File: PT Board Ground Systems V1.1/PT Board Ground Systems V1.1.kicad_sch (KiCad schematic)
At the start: 9 parts, among them J1 POWER IN, J2 OUT CHAN A, J3 OUT CHAN B

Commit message: Changed all the things to 5mm pitch
yuck big board be like
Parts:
- J1: footprint TerminalBlock_Phoenix:TerminalBlock_Phoenix_MPT-0,5-2-2.54_1x02_P2.54mm_Horizontal -> TerminalBlock_Phoenix:TerminalBlock_Phoenix_PT-1,5-2-5.0-H_1x02_P5.00mm_Horizontal
- J2, J3: footprint TerminalBlock_Phoenix:TerminalBlock_Phoenix_MPT-0,5-8-2.54_1x08_P2.54mm_Horizontal -> TerminalBlock_Phoenix:TerminalBlock_Phoenix_PT-1,5-8-5.0-H_1x08_P5.00mm_Horizontal

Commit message: Woek
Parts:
- J1: footprint TerminalBlock_Phoenix:TerminalBlock_Phoenix_PT-1,5-2-5.0-H_1x02_P5.00mm_Horizontal -> TerminalBlock_Phoenix:TerminalBlock_Phoenix_PT-1,5-2-3.5-H_1x02_P3.50mm_Horizontal
- J2, J3: footprint TerminalBlock_Phoenix:TerminalBlock_Phoenix_PT-1,5-8-5.0-H_1x08_P5.00mm_Horizontal -> TerminalBlock_Phoenix:TerminalBlock_Phoenix_PT-1,5-8-3.5-H_1x08_P3.50mm_Horizontal
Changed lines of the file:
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@@
       (effects (font (size 1.27 1.27)))
     )
-    (property "Footprint" "TerminalBlock_Phoenix:TerminalBlock_Phoenix_PT-1,5-2-5.0-H_1x02_P5.00mm_Horizontal" (at 20.32 30.48 0)
+    (property "Footprint" "TerminalBlock_Phoenix:TerminalBlock_Phoenix_PT-1,5-2-3.5-H_1x02_P3.50mm_Horizontal" (at 20.32 30.48 0)
       (effects (font (size 1.27 1.27)) hide)
     )
@@
       (effects (font (size 1.27 1.27)))
     )
-    (property "Footprint" "TerminalBlock_Phoenix:TerminalBlock_Phoenix_PT-1,5-8-5.0-H_1x08_P5.00mm_Horizontal" (at 53.34 19.685 0)
+    (property "Footprint" "TerminalBlock_Phoenix:TerminalBlock_Phoenix_PT-1,5-8-3.5-H_1x08_P3.50mm_Horizontal" (at 53.34 19.685 0)
       (effects (font (size 1.27 1.27)) hide)
     )
@@
       (effects (font (size 1.27 1.27)))
     )
-    (property "Footprint" "TerminalBlock_Phoenix:TerminalBlock_Phoenix_PT-1,5-8-5.0-H_1x08_P5.00mm_Horizontal" (at 74.93 19.685 0)
-      (effects (font (size 1.27 1.27)) hide)
-    )
+    (property "Footprint" "TerminalBlock_Phoenix:TerminalBlock_Phoenix_PT-1,5-8-3.5-H_1x08_P3.50mm_Horizontal" (at 74.93 19.685 0)
+      (effects (font (size 1.27 1.27)) hide)
+    )

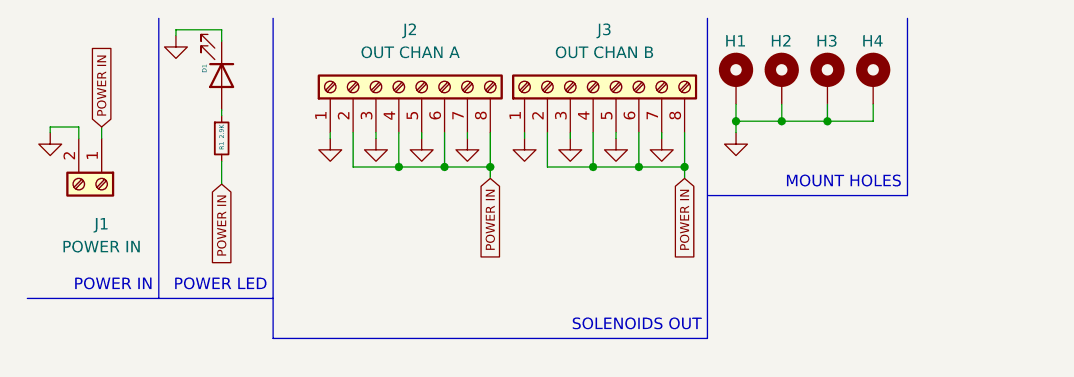
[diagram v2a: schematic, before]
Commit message: Revions and new board
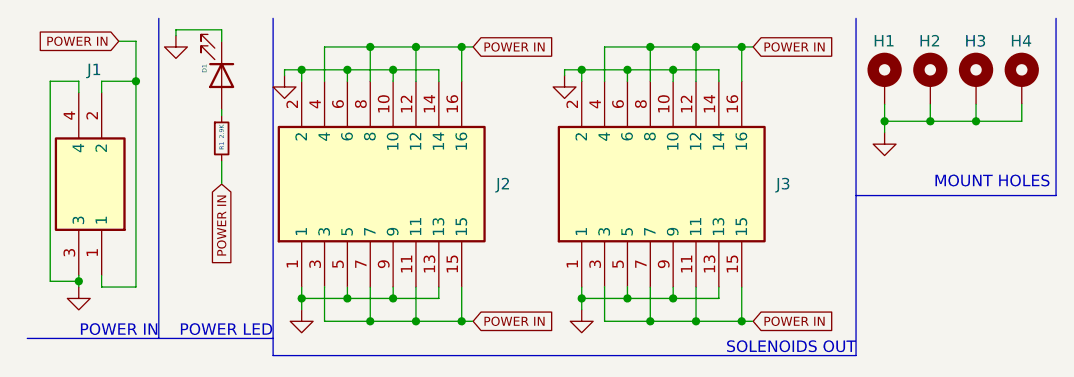
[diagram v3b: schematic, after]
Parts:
- removed J1: POWER IN, TerminalBlock_Phoenix:TerminalBlock_Phoenix_PT-1,5-2-3.5-H_1x02_P3.50mm_Horizontal, symbol Connector:Screw_Terminal_01x02
- removed J2: OUT CHAN A, TerminalBlock_Phoenix:TerminalBlock_Phoenix_PT-1,5-8-3.5-H_1x08_P3.50mm_Horizontal, symbol Connector:Screw_Terminal_01x08
- removed J3: OUT CHAN B, TerminalBlock_Phoenix:TerminalBlock_Phoenix_PT-1,5-8-3.5-H_1x08_P3.50mm_Horizontal, symbol Connector:Screw_Terminal_01x08
- added J1: TBLH10V-350-02BK, RHDR4W80P550X350_2X2_770X850X1420P, symbol TBLH10V-350-02BK:TBLH10V-350-02BK
- added J2, J3: TBLH10V-350-08BK, RHDR16W80P550X350_2X8_2870X850X1420P, symbol TBLH10V-350-08BK:TBLH10V-350-08BK
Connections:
- net GND: now also J1.3, J1.4, J2.1, J2.10, J2.13, J2.14, J2.2, J2.5, J2.6, J2.9, J3.1, J3.10, J3.13, J3.14, J3.2, J3.5, J3.6, J3.9
- net POWER IN: now also J1.1, J1.2, J2.11, J2.12, J2.15, J2.16, J2.3, J2.4, J2.7, J2.8, J3.11, J3.12, J3.15, J3.16, J3.3, J3.4, J3.7, J3.8
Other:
- moved on the sheet: H1, H2, H3, H4
